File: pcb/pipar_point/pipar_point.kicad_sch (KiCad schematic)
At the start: 40 parts, among them SW1 SW_Wuerth_450301014042, U1 Seeeduino Xiao nRF52840

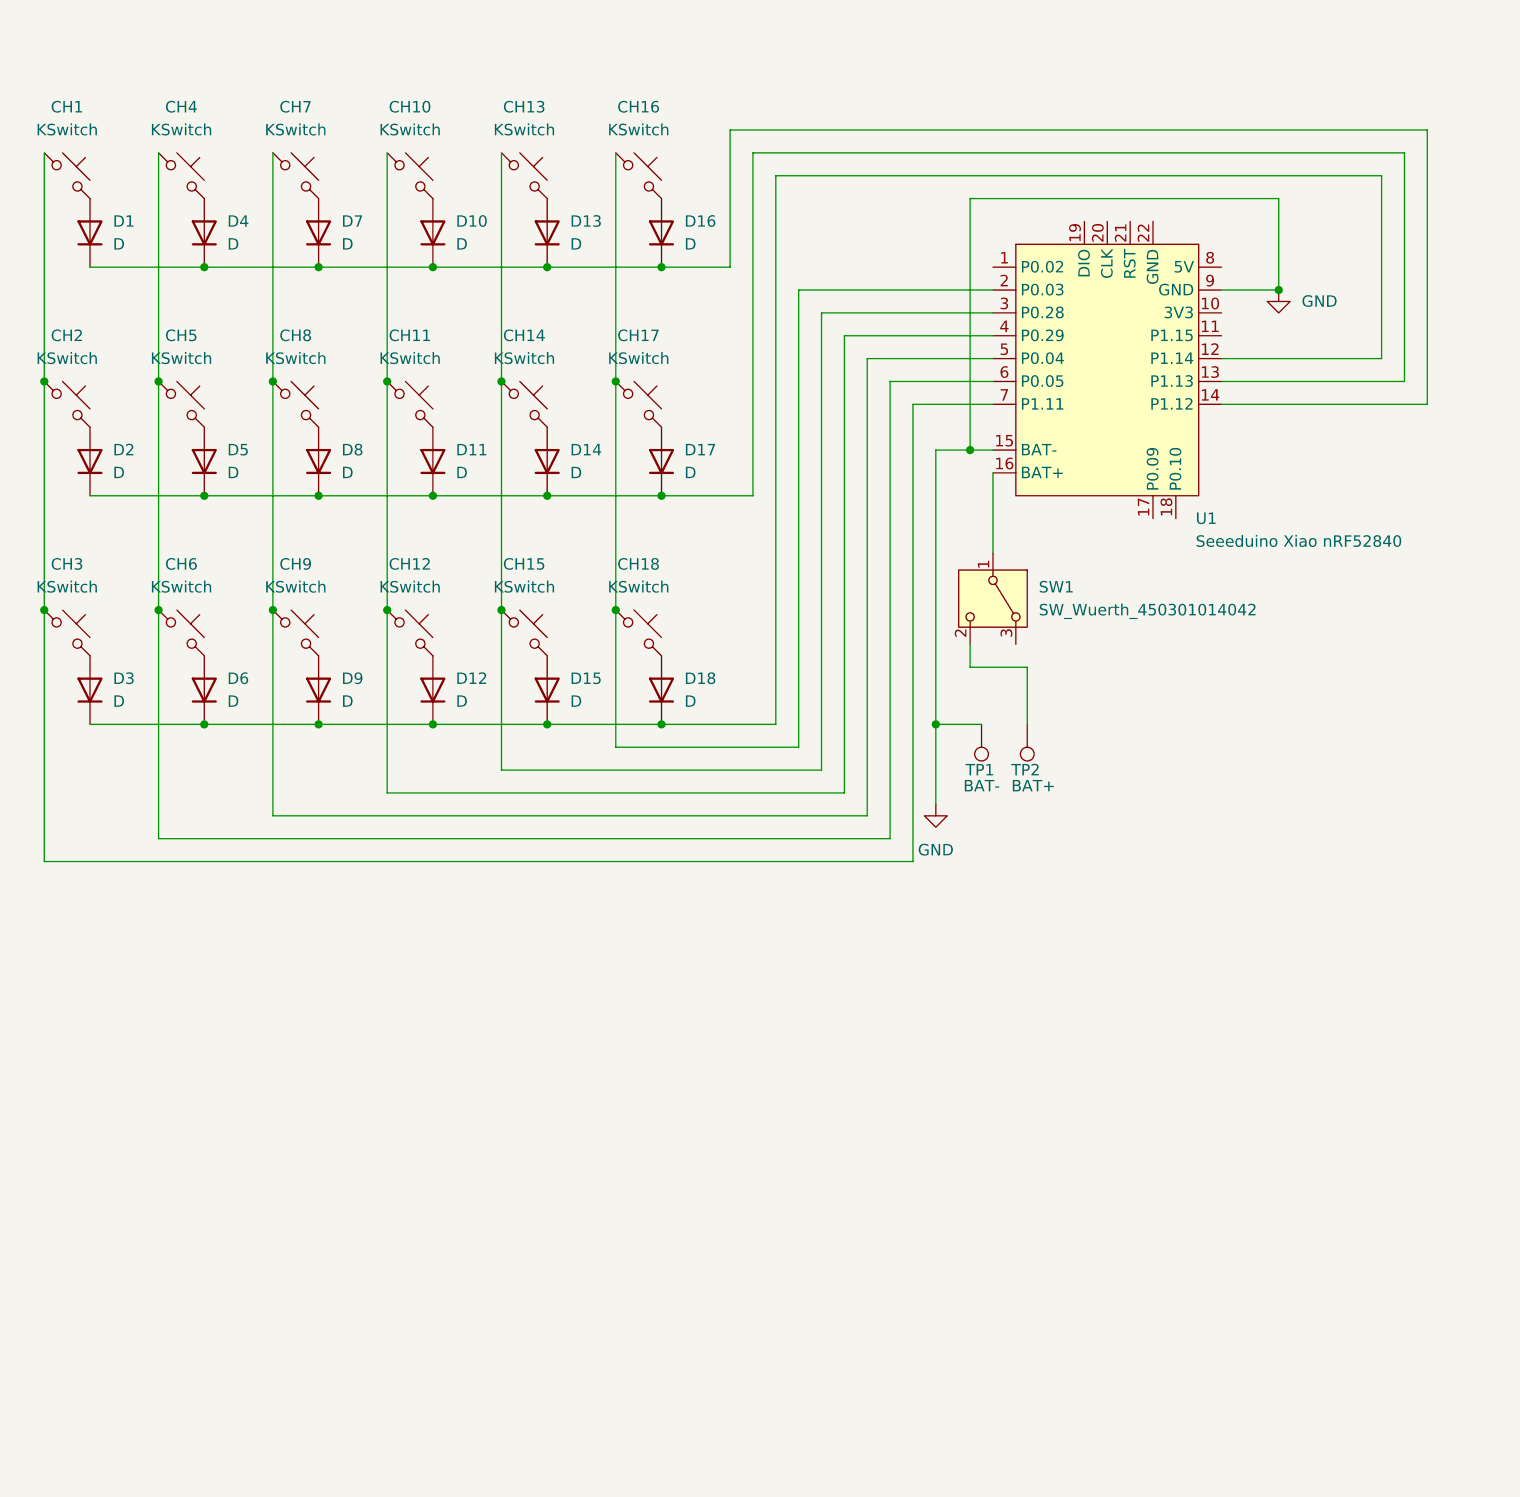
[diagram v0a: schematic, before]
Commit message: implements schematic
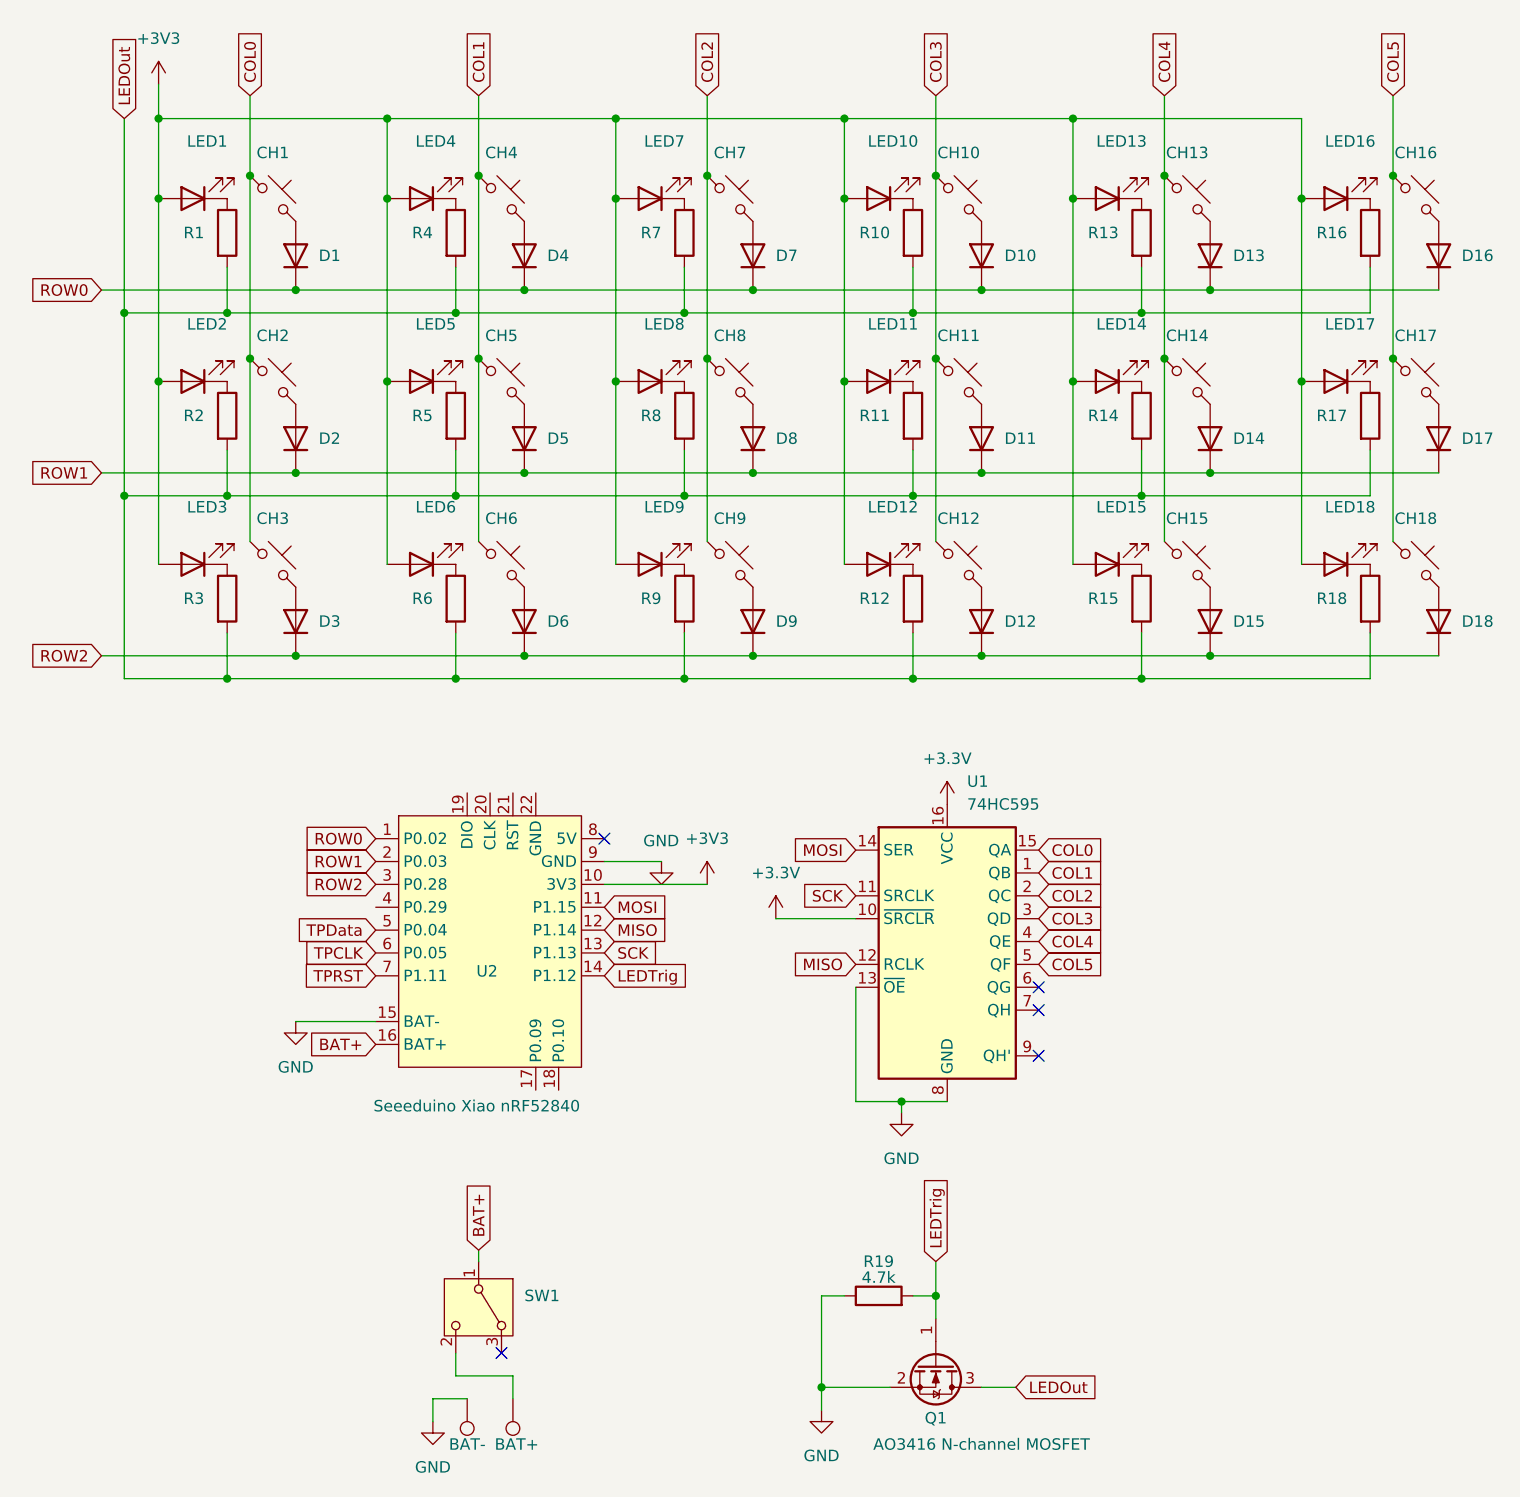
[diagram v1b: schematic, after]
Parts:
- added LED1, LED10, LED11, LED12, LED13, LED14, LED15, LED16, LED17, LED18, LED2, LED3, LED4, LED5, LED6, LED7, LED8, LED9: ~, LED_SMD:LED_1206_3216Metric, symbol LED:IR26-21C_L110_TR8
- added Q1: AO3416 N-channel MOSFET, Package_TO_SOT_SMD:SOT-23, symbol Device:Q_NMOS_GSD
- added R1, R10, R11, R12, R13, R14, R15, R16, R17, R18, R2, R3, R4, R5, R6, R7, R8, R9: 10m_1206_250mW, Resistor_SMD:R_1206_3216Metric, symbol PCM_4ms_Resistor:10m_1206_250mW
- added R19: 4.7k, Resistor_SMD:R_1206_3216Metric, symbol PCM_4ms_Resistor:10m_1206_250mW
- added U1: 74HC595, symbol 74xx:74HC595
- renumbered U1 to U2
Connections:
- net GND: now also Q1.2 (S), R19.1, U1.13 (~{OE}), U1.8 (GND)
- net COL4: now reaches CH13.1, CH14.1, CH15.1
- net COL4: now also U1.4 (QE); no longer U2.3 (P0.28)
- net COL2: now reaches CH7.1, CH8.1, CH9.1
- net COL2: now also U1.2 (QC); no longer U2.5 (P0.04)
- net COL5: now reaches CH16.1, CH17.1, CH18.1
- net COL5: now also U1.5 (QF); no longer U2.2 (P0.03)
- net ROW1: now reaches D11.1 (K), D14.1 (K), D17.1 (K), D2.1 (K), D5.1 (K), D8.1 (K)
- net ROW1: now also U2.2 (P0.03); no longer U2.13 (P1.13)
- net COL0: now reaches CH1.1, CH2.1, CH3.1
- net COL0: now also U1.15 (QA); no longer U2.7 (P1.11)
- net COL1: now reaches CH4.1, CH5.1, CH6.1
- net COL1: now also U1.1 (QB); no longer U2.6 (P0.05)
- net COL3: now reaches CH10.1, CH11.1, CH12.1
- net COL3: now also U1.3 (QD); no longer U2.4 (P0.29)
- net ROW2: now reaches D12.1 (K), D15.1 (K), D18.1 (K), D3.1 (K), D6.1 (K), D9.1 (K)
- net ROW2: now also U2.3 (P0.28); no longer U2.12 (P1.14)
- net ROW0: now reaches U2.1 (P0.02)
- net ROW0: now also D1.1 (K), D10.1 (K), D13.1 (K), D16.1 (K), D4.1 (K), D7.1 (K)
- net +3V3: now reaches U2.10 (3V3)
- net +3V3: now also LED1.2 (A), LED10.2 (A), LED11.2 (A), LED12.2 (A), LED13.2 (A), LED14.2 (A), LED15.2 (A), LED16.2 (A), LED17.2 (A), LED18.2 (A), LED2.2 (A), LED3.2 (A), LED4.2 (A), LED5.2 (A), LED6.2 (A), LED7.2 (A), LED8.2 (A), LED9.2 (A)
- net MOSI: now reaches U2.11 (P1.15)
- net MOSI: now also U1.14 (SER)
- net BAT+: now reaches SW1.1 (B), U2.16 (BAT+)
- new net: LED7.1 (K), R7.1
- new net: LED10.1 (K), R10.1
- new net: LED13.1 (K), R13.1
- new net: LED16.1 (K), R16.1
- new net: LED9.1 (K), R9.1
- new net: LED15.1 (K), R15.1
- new net: LED12.1 (K), R12.1
- new net: LED6.1 (K), R6.1
- new net: LED1.1 (K), R1.1
- new net: LED5.1 (K), R5.1
- new net: LED18.1 (K), R18.1
- new net: LED8.1 (K), R8.1
- new net: LED11.1 (K), R11.1
- new net: LED17.1 (K), R17.1
- new net: LED4.1 (K), R4.1
- new net: LED3.1 (K), R3.1
- new net: LED14.1 (K), R14.1
- new net: LED2.1 (K), R2.1
- new net  SCK: U1.11 (SRCLK), U2.13 (P1.13)
- new net +3.3V: U1.10 (~{SRCLR}), U1.16 (VCC)
- new net LEDOut: Q1.3 (D), R1.2, R10.2, R11.2, R12.2, R13.2, R14.2, R15.2, R16.2, R17.2, R18.2, R2.2, R3.2, R4.2, R5.2, R6.2, R7.2, R8.2, R9.2
- new net LEDTrig: Q1.1 (G), R19.2, U2.14 (P1.12)
- new net MISO: U1.12 (RCLK), U2.12 (P1.14)
- new net TPCLK: U2.6 (P0.05)
- new net TPData: U2.5 (P0.04)
- new net TPRST: U2.7 (P1.11)
- no-connect marks 0 -> 5
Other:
- moved on the sheet: SW1, U2
